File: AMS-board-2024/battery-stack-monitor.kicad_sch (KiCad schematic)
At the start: 68 parts, among them Q115 STD7ANM60N, Q116 STD7ANM60N, Q117 2N7002K-AU, Q118 STD7ANM60N, U23 LM25180-Q1, U24 LTC2949, U25 NCV8711BMTW500TBG, U26 NV24C16SNVLT3G, Y2 ABLS-4.000MHZ-K4T

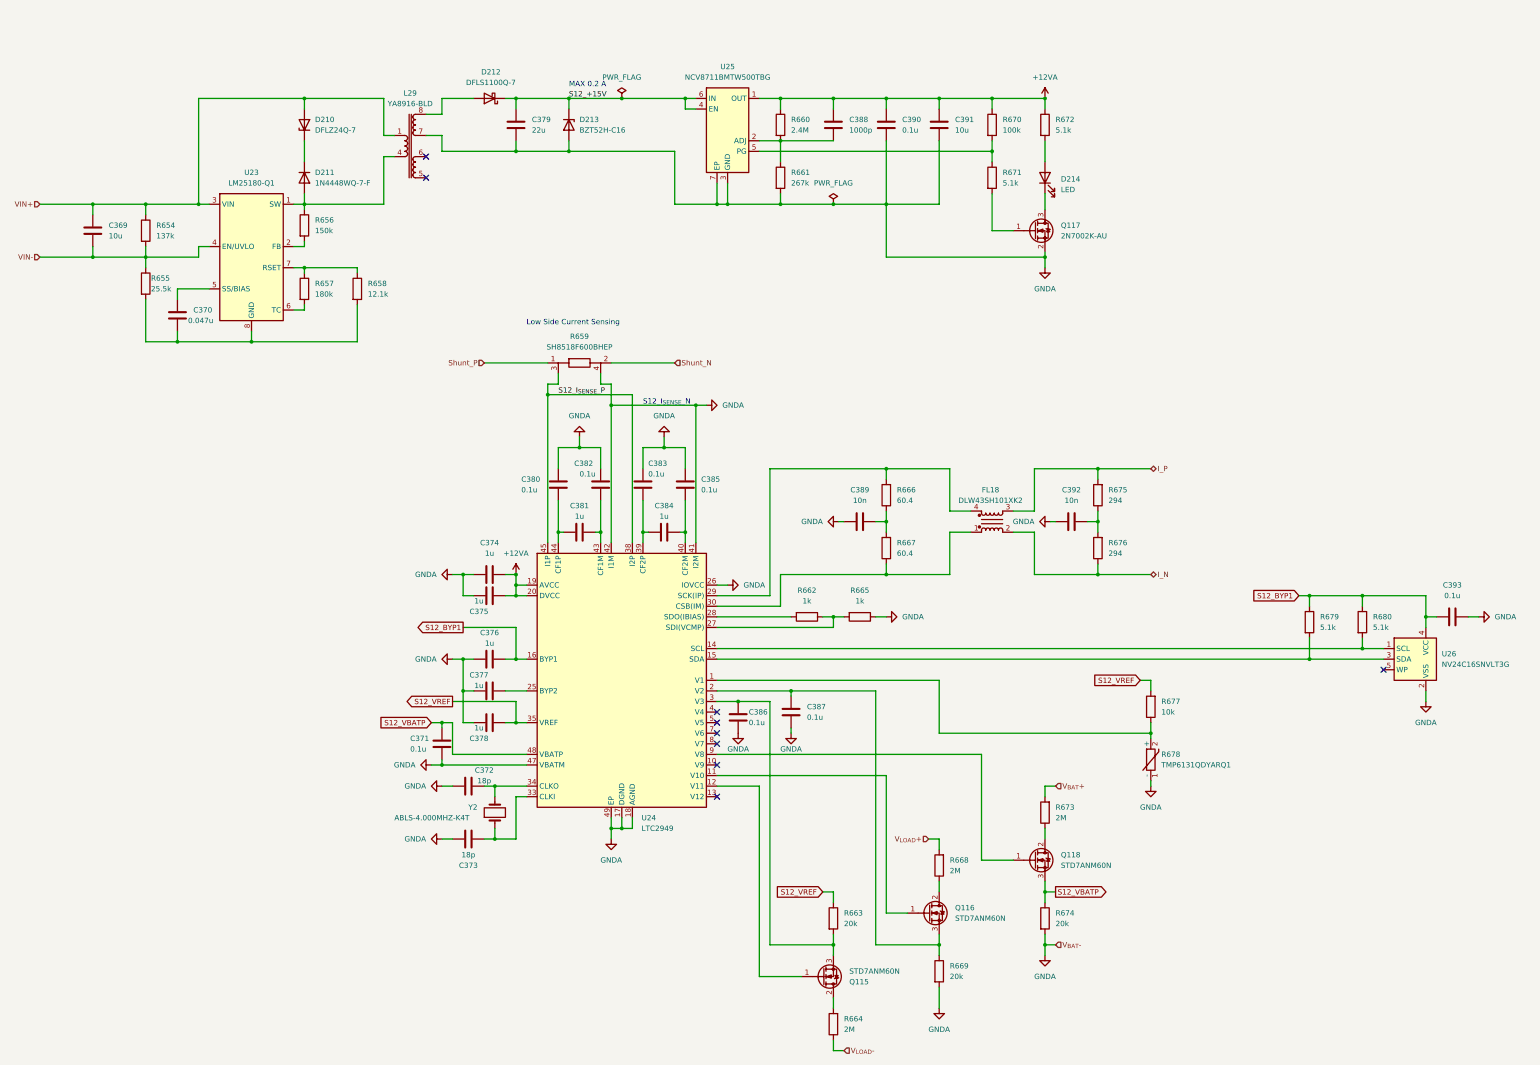
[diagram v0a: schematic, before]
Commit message: 階層シート内の電源シンボル修正
階層シート内で電源シンボルをなるべく使わないようにする
修正途中
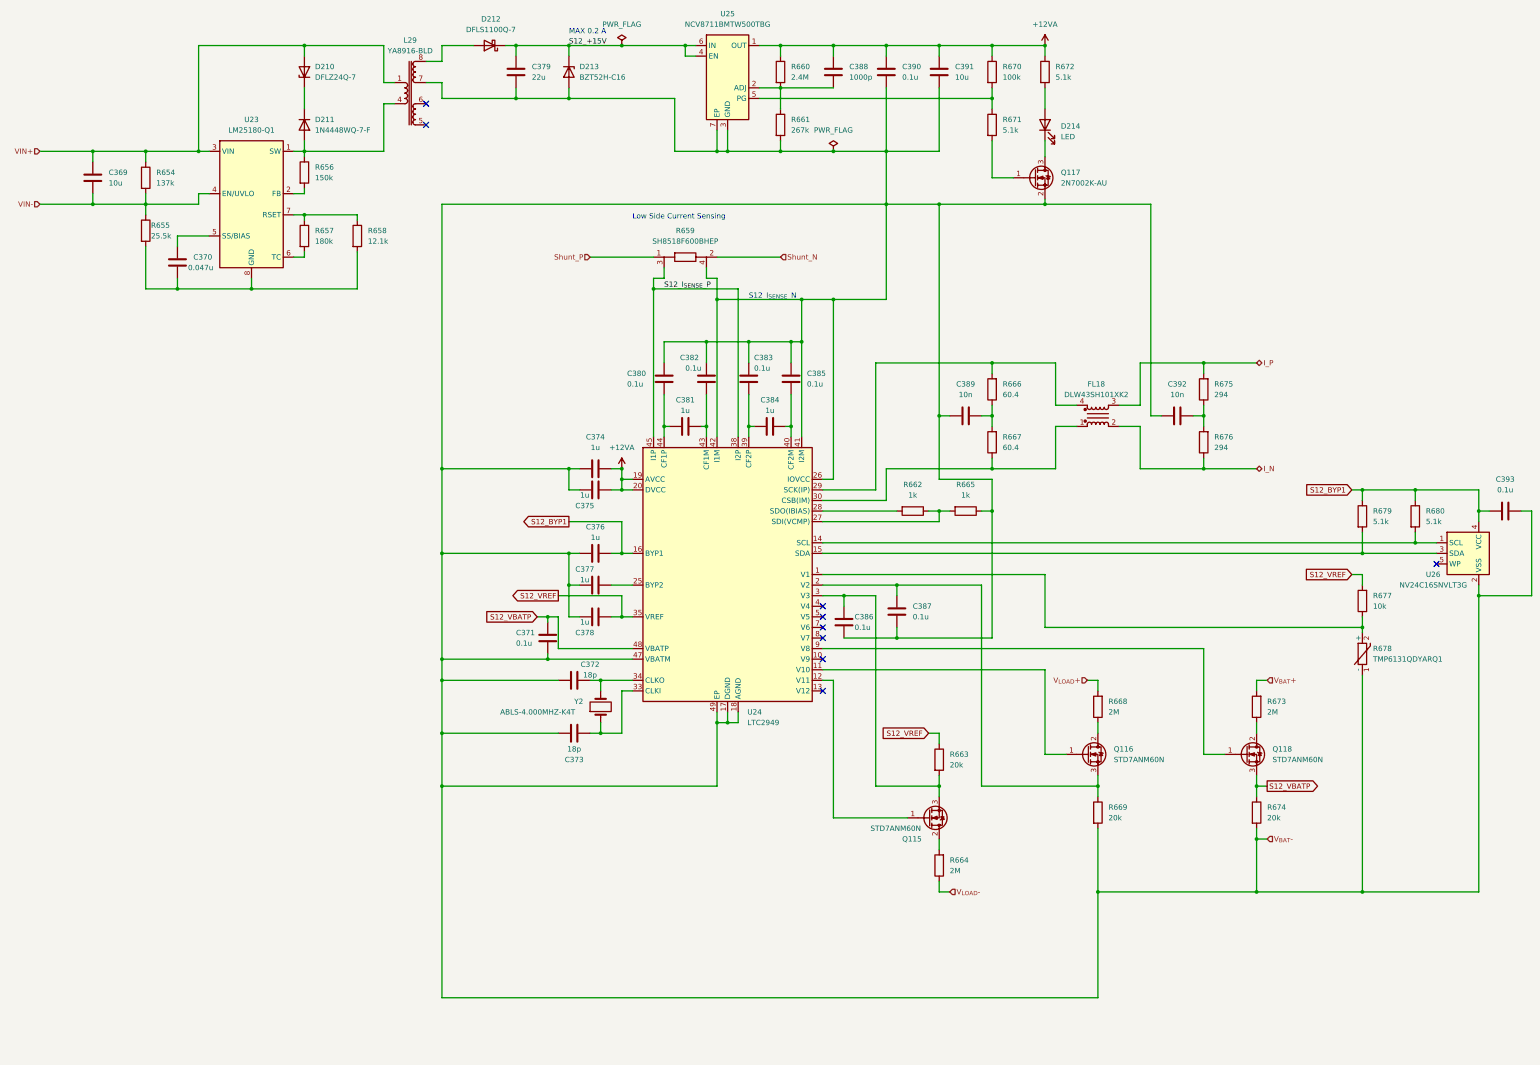
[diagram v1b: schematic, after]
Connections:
- net GNDA renamed V_{BAT}-
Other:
- moved on the sheet: C369, C370, C371, C372, C373, C374, C375, C376, C377, C378, C379, C380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
